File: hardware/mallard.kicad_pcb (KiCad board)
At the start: 4 copper layers, 101.6 x 101.6 mm, 86 parts, among them J1 USB_A, J2 Conn_02x03_Odd_Even, J3 Conn_01x03, J4 Conn_01x03, J5 Conn_01x03, J6 Conn_01x03, SW1 RESET Switch, U1 TMP235, U10 LTC1983ES6-3, U11 STM32L4Q5xx, U12 LTC3529EDCB, U2 TMP235, U3 TMP235, U4 BQ24210DQCT, U5 TMUX1309, U6 TMUX1309, U7 LMP7721, U8 TPS71710DRVR, U9 LMV554

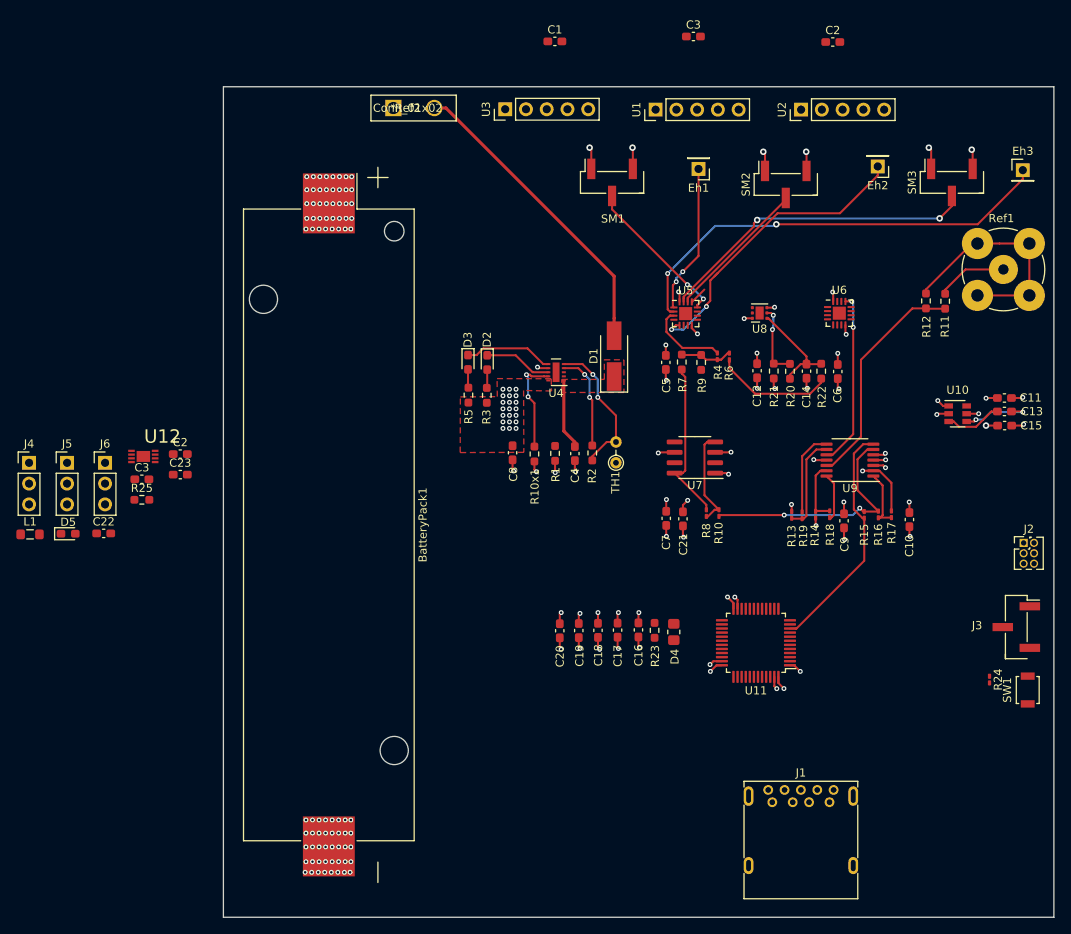
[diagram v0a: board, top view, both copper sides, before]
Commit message: Schematic and Layout Finished
Needs review
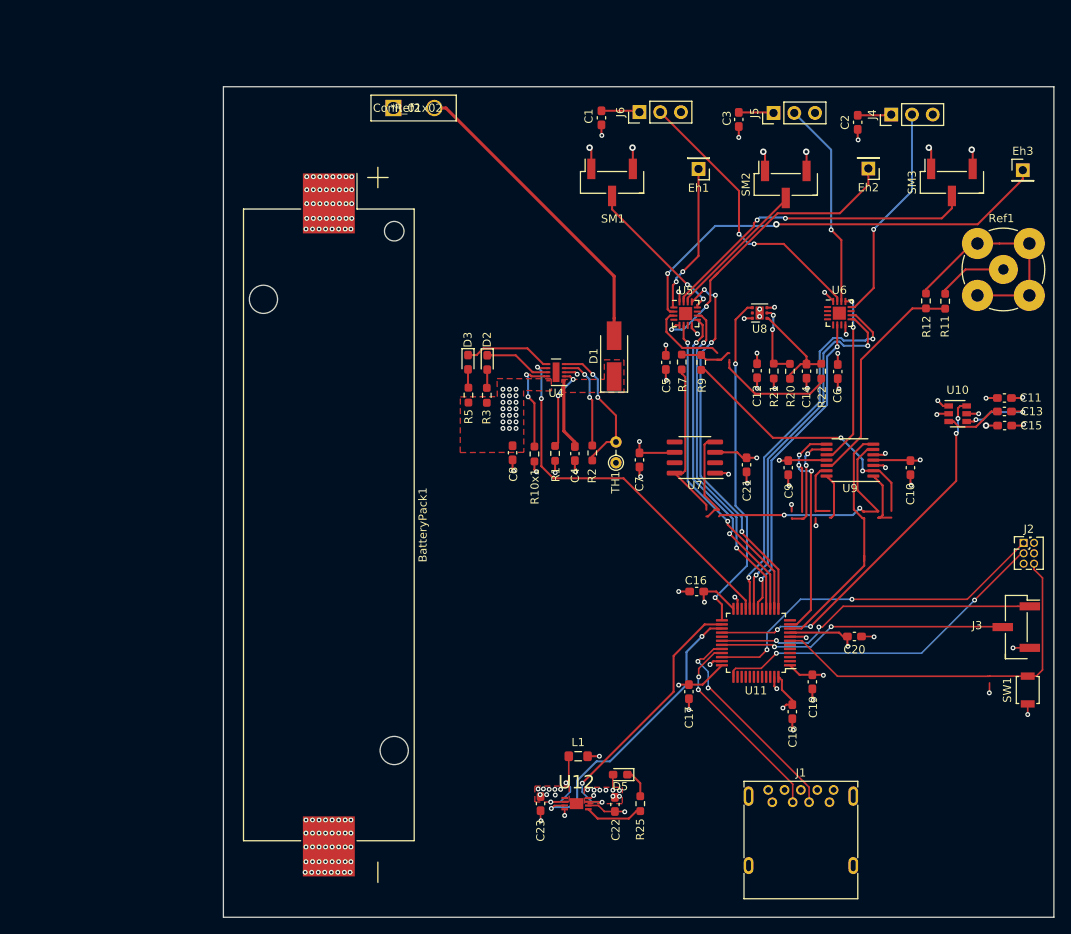
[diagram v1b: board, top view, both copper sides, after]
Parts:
- removed the C2 at (34.9, 78.7)
- removed the C2 at (114.8, 28.3)
- removed the C3 at (30.2, 81.8)
- removed D4: Orange, Resistor_SMD:R_0805_2012Metric_Pad1.20x1.40mm_HandSolder
- removed R10, R19: 20k, Resistor_SMD:R_0201_0603Metric_Pad0.64x0.40mm_HandSolder
- removed R13, R17, R24, R4, R6, R8: 10k, Resistor_SMD:R_0201_0603Metric_Pad0.64x0.40mm_HandSolder
- removed R14: 1k, Resistor_SMD:R_0201_0603Metric_Pad0.64x0.40mm_HandSolder
- removed R15: 30k, Resistor_SMD:R_0201_0603Metric_Pad0.64x0.40mm_HandSolder
- removed R16: 20k DNI, Resistor_SMD:R_0201_0603Metric_Pad0.64x0.40mm_HandSolder
- removed R18: 9.1k, Resistor_SMD:R_0201_0603Metric_Pad0.64x0.40mm_HandSolder
- removed R23: 680, Resistor_SMD:R_0603_1608Metric_Pad0.98x0.95mm_HandSolder
- removed U1, U2, U3: TMP235, Connector_PinHeader_2.54mm:PinHeader_1x05_P2.54mm_Vertical
- added C2: 1uF, Capacitor_SMD:C_0603_1608Metric_Pad1.08x0.95mm_HandSolder, F.Cu at (117.8, 38.1)
- moved J4 113.8 mm to (121.9, 37.2), turned to 90 degrees
- moved J5 96.4 mm to (107.5, 37.0), turned to 90 degrees
- moved J6 78.2 mm to (91.1, 36.9), turned to 90 degrees
- moved D5 73.7 mm to (88.8, 118.0), turned to 180 degrees
- moved L1 72.3 mm to (83.6, 115.7), turned to 180 degrees
- moved R25 71.4 mm to (91.2, 121.5), turned to 90 degrees
- moved C22 70.8 mm to (88.1, 121.6), turned to 270 degrees
- moved U12 67.9 mm to (83.4, 121.5)
- moved C23 59.7 mm to (79.0, 121.5), turned to 270 degrees
- moved C20 36.1 mm to (117.4, 101.0), turned to 0 degrees
- moved C19 29.3 mm to (112.2, 106.6)
- moved C18 25.8 mm to (109.8, 110.2)
- moved C3 11.6 mm to (103.2, 37.8), turned to 270 degrees
- moved C17 11.5 mm to (97.2, 107.8)
- moved C1 11.0 mm to (86.5, 37.6), turned to 270 degrees
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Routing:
- net MUX2_A1: track 0.00 -> 46.9 mm, vias 0 -> 2
- net -3V3_SHDN_L: track 0.00 -> 46.5 mm, vias 0 -> 4
- net /RESET_L: track 0.00 -> 46.4 mm
- net MUX2_A0: track 0.00 -> 45.4 mm, vias 0 -> 2
- net Charge_EN: track 1.38 -> 46.5 mm, vias 1 -> 2
- net Moisture_Sense: track 2.16 -> 46.9 mm, vias 0 -> 4
- net /SWDIO: track 0.00 -> 43.9 mm, vias 0 -> 2
- net /SWCLK: track 0.00 -> 42.2 mm, vias 0 -> 2
- net +1V0_EN: track 0.00 -> 42.0 mm, vias 0 -> 2
- net +3V3: track 37.9 -> 79.2 mm, vias 85 -> 90
- net MUX1_A1: track 0.00 -> 40.6 mm, vias 0 -> 2
- net MUX1_A0: track 0.00 -> 40.3 mm, vias 0 -> 2
- net USART1_TX: track 0.00 -> 40.0 mm, vias 0 -> 2
- net MUX1_EN: track 0.00 -> 39.3 mm, vias 0 -> 2
- net MUX2_EN: track 0.00 -> 38.9 mm, vias 0 -> 2
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- added copper zone on F.Cu, net +5V
- added copper zone on Power, net +5V
